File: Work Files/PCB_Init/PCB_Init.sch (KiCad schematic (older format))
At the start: 35 parts

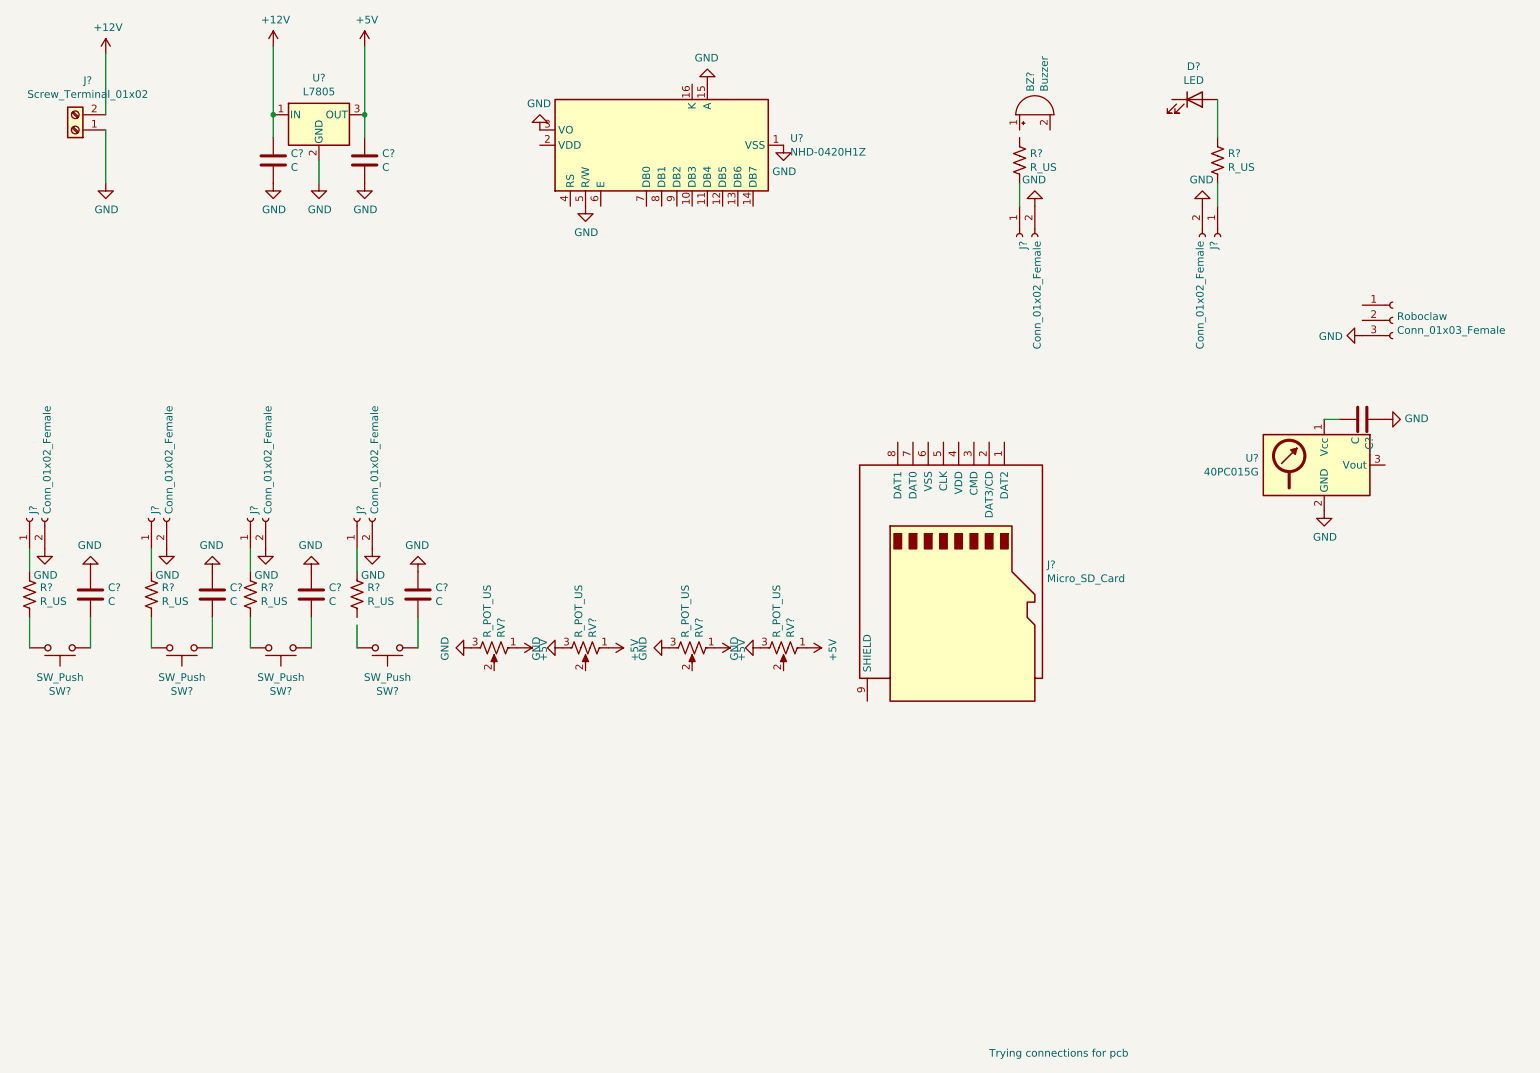
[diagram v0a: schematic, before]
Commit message: Started designing PCB
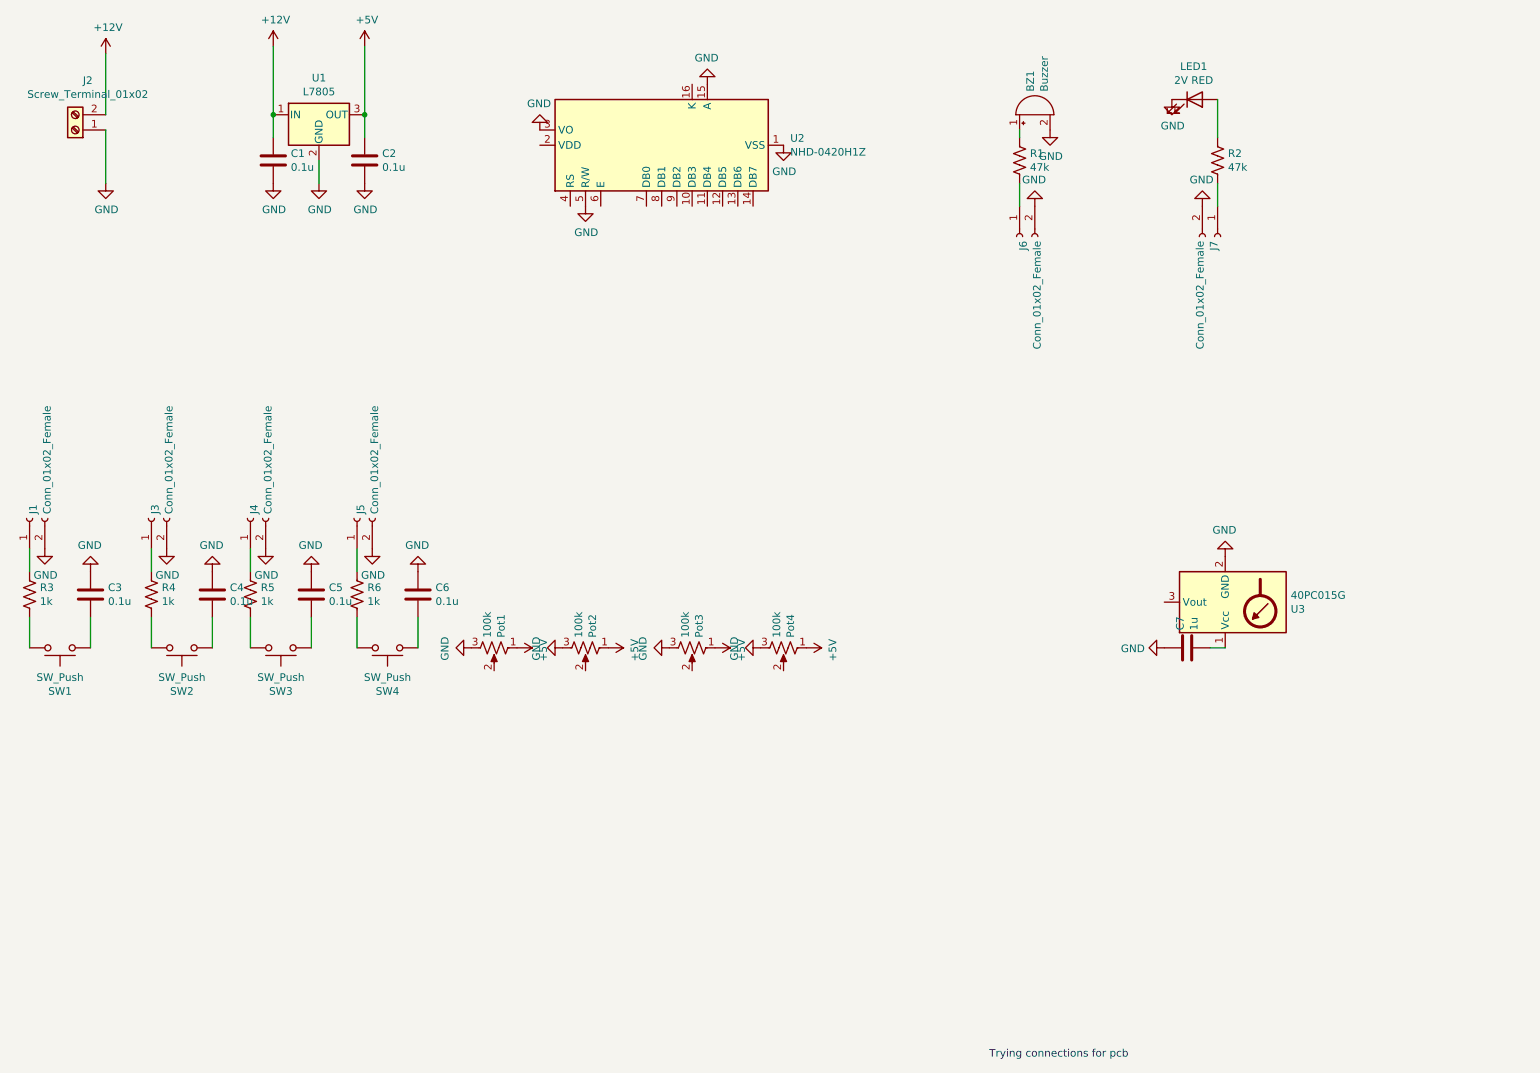
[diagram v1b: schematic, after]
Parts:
- removed J?: Micro_SD_Card, symbol Connector:Micro_SD_Card
- removed Roboclaw: Conn_01x03_Female, symbol Connector:Conn_01x03_Female
- BZ1: renamed from BZ?; footprint (none) -> Buzzer_Beeper:Buzzer_12x9.5RM7.6
- C1, C2, C3, C4, C5, C6: renamed from C?; value C -> 0.1u; footprint (none) -> Capacitor_THT:CP_Radial_D8.0mm_P5.00mm; Spice_Model (none) -> 0.1u; Spice_Netlist_Enabled (none) -> Y; Spice_Primitive (none) -> C
- C7: renamed from C?; value C -> 1u; footprint (none) -> Capacitor_THT:CP_Radial_D8.0mm_P5.00mm; Spice_Model (none) -> 1u; Spice_Netlist_Enabled (none) -> Y; Spice_Primitive (none) -> C
- J1, J3, J4, J5, J6, J7: renamed from J?; footprint (none) -> Connector_PinHeader_1.27mm:PinHeader_1x02_P1.27mm_Vertical
- J2: renamed from J?; footprint (none) -> TerminalBlock:TerminalBlock_Altech_AK300-2_P5.00mm
- LED1: renamed from D?; value LED -> 2V RED; footprint (none) -> LED_THT:LED_D3.0mm
- Pot1, Pot2, Pot3, Pot4: renamed from RV?; value R_POT_US -> 100k; footprint (none) -> Potentiometer_THT:Potentiometer_Bourns_3296W_Vertical; Spice_Model (none) -> 100k; Spice_Netlist_Enabled (none) -> Y; Spice_Primitive (none) -> R
- R1, R2: renamed from R?; value R_US -> 47k; footprint (none) -> Resistor_THT:R_Axial_DIN0204_L3.6mm_D1.6mm_P5.08mm_Horizontal; Spice_Model (none) -> 47k; Spice_Netlist_Enabled (none) -> Y; Spice_Primitive (none) -> R
- R3, R4, R5, R6: renamed from R?; value R_US -> 1k; footprint (none) -> Resistor_THT:R_Axial_DIN0204_L3.6mm_D1.6mm_P5.08mm_Horizontal; Spice_Model (none) -> 1k; Spice_Netlist_Enabled (none) -> Y; Spice_Primitive (none) -> R
- SW1, SW2, SW3, SW4: renamed from SW?; footprint (none) -> Button_Switch_THT:SW_PUSH-12mm
- U1: renamed from U?; footprint (none) -> Package_TO_SOT_THT:TO-3P-3_Vertical
- U3: renamed from U?; footprint (none) -> Sensor_Pressure:Honeywell_40PCxxxG1A
- gave numbers to parts that had none: 1
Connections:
- wire segments 23 -> 24
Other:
- moved on the sheet: C7, U3

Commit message: Started designing PCB2
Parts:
- J1, J3, J4, J5, J6, J7: footprint Connector_PinHeader_1.27mm:PinHeader_1x02_P1.27mm_Vertical -> Connector_PinHeader_2.54mm:PinHeader_1x02_P2.54mm_Vertical
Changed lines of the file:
@@
 F 0 "J3" H 1828 3876 50  0000 L CNN
 F 1 "Conn_01x02_Female" H 1828 3785 50  0000 L CNN
-F 2 "Connector_PinHeader_1.27mm:PinHeader_1x02_P1.27mm_Vertical" H 1800 3900 50  0001 C CNN
+F 2 "Connector_PinHeader_2.54mm:PinHeader_1x02_P2.54mm_Vertical" H 1800 3900 50  0001 C CNN
 F 3 "~" H 1800 3900 50  0001 C CNN
 	1    1800 3900
@@
 F 0 "J4" H 2478 3876 50  0000 L CNN
 F 1 "Conn_01x02_Female" H 2478 3785 50  0000 L CNN
-F 2 "Connector_PinHeader_1.27mm:PinHeader_1x02_P1.27mm_Vertical" H 2450 3900 50  0001 C CNN
+F 2 "Connector_PinHeader_2.54mm:PinHeader_1x02_P2.54mm_Vertical" H 2450 3900 50  0001 C CNN
 F 3 "~" H 2450 3900 50  0001 C CNN
 	1    2450 3900
@@
 F 0 "J5" H 3178 3876 50  0000 L CNN
 F 1 "Conn_01x02_Female" H 3178 3785 50  0000 L CNN
-F 2 "Connector_PinHeader_1.27mm:PinHeader_1x02_P1.27mm_Vertical" H 3150 3900 50  0001 C CNN
+F 2 "Connector_PinHeader_2.54mm:PinHeader_1x02_P2.54mm_Vertical" H 3150 3900 50  0001 C CNN
 F 3 "~" H 3150 3900 50  0001 C CNN
 	1    3150 3900
@@
 F 0 "J6" H 7528 2026 50  0000 L CNN
 F 1 "Conn_01x02_Female" H 7528 1935 50  0000 L CNN
-F 2 "Connector_PinHeader_1.27mm:PinHeader_1x02_P1.27mm_Vertical" H 7500 2050 50  0001 C CNN
+F 2 "Connector_PinHeader_2.54mm:PinHeader_1x02_P2.54mm_Vertical" H 7500 2050 50  0001 C CNN
 F 3 "~" H 7500 2050 50  0001 C CNN
 	1    7500 2050
@@
 F 0 "J1" H 1028 3876 50  0000 L CNN
 F 1 "Conn_01x02_Female" H 1028 3785 50  0000 L CNN
-F 2 "Connector_PinHeader_1.27mm:PinHeader_1x02_P1.27mm_Vertical" H 1000 3900 50  0001 C CNN
+F 2 "Connector_PinHeader_2.54mm:PinHeader_1x02_P2.54mm_Vertical" H 1000 3900 50  0001 C CNN
 F 3 "~" H 1000 3900 50  0001 C CNN
 	1    1000 3900
@@
 F 0 "J7" H 8828 2026 50  0000 L CNN
 F 1 "Conn_01x02_Female" H 8828 1935 50  0000 L CNN
-F 2 "Connector_PinHeader_1.27mm:PinHeader_1x02_P1.27mm_Vertical" H 8800 2050 50  0001 C CNN
+F 2 "Connector_PinHeader_2.54mm:PinHeader_1x02_P2.54mm_Vertical" H 8800 2050 50  0001 C CNN
 F 3 "~" H 8800 2050 50  0001 C CNN
 	1    8800 2050
